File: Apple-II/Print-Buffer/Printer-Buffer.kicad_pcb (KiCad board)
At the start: 2 copper layers, 133 x 75 mm, 12 parts, among them J1 Apple-II-Expansion-Slot, J2 CONN_13X2, U1 HM6116, U2 74LS374, U3 74125, U4 74121, U5 74LS138, U6 74LS02, U7 7404

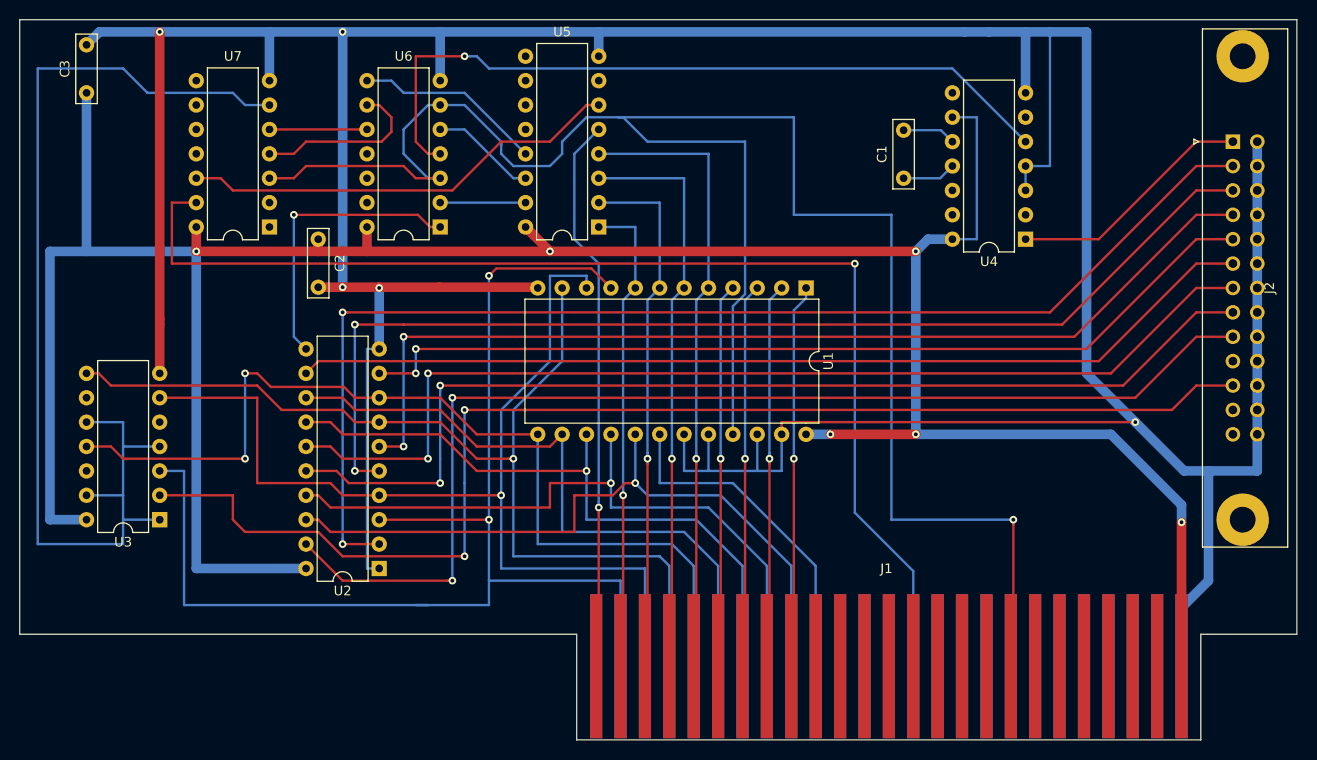
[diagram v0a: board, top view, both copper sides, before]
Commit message: PCB tweaks and some images
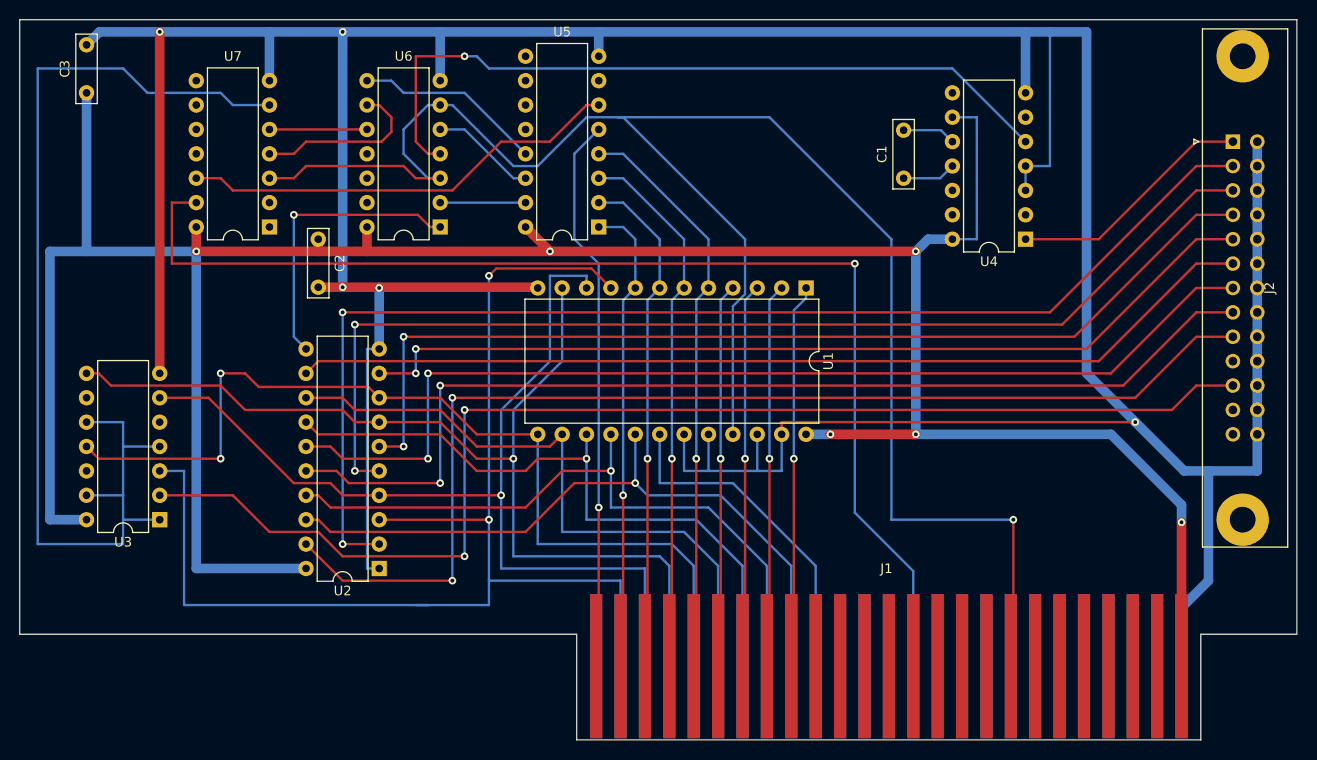
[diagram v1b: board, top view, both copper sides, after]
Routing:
- net R~W: track 197.4 -> 182.1 mm
- net D1: track 105.2 -> 100.0 mm
- net A3: track 62.9 -> 57.7 mm
- net A2: track 57.8 -> 54.1 mm
- net D7: track 71.9 -> 69.7 mm
- net A1: track 52.7 -> 50.5 mm
- net Printer-Busy: track 132.2 -> 130.7 mm
- net D6: track 69.1 -> 68.1 mm
- net A0: track 47.6 -> 46.9 mm
- net D5: track 66.3 -> 66.9 mm

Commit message: upgraded to KiCad 6.0
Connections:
- net R~W renamed R~{W}
- net ~Data-Strobe renamed ~{Data-Strobe}
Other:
- net class Default removed
